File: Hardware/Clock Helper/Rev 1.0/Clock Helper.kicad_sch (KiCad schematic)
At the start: 16 parts, among them J1 IO, SW1 CYCLE/INSTR, SW2 RUN/STOP, SW3 STEP, U1 74HC74

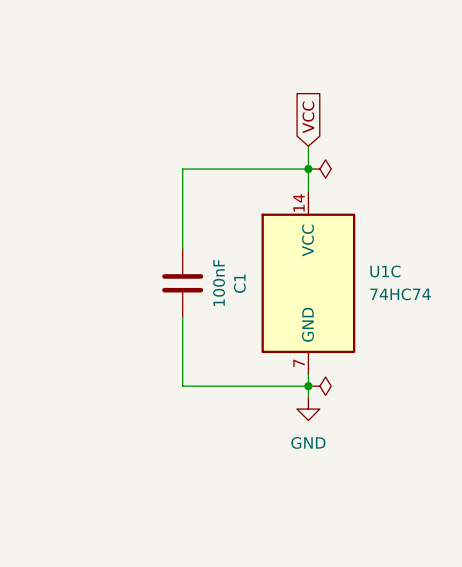
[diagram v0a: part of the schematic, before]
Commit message: Project restructuring
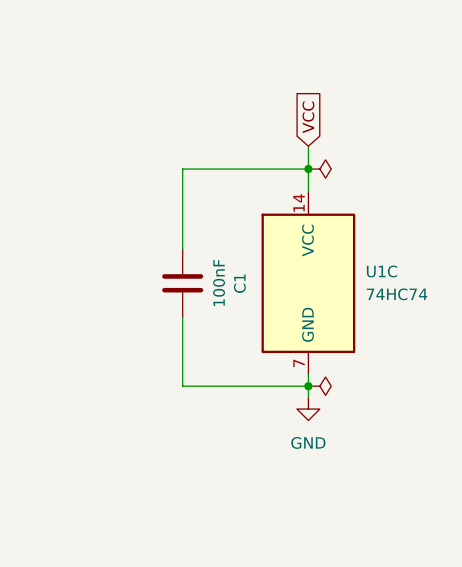
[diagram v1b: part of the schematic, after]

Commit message: Add BOMs
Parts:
- C1: LCSC C49678 -> (none)
- J1: now in the parts list
- R3, R4, R5: LCSC C17513 -> (none)
- SW1, SW2: LCSC (none) -> XKB5858-Z; MPN XKB5858-Z -> (none)
- SW3: LCSC (none) -> XKB5858-W; MPN XKB5858-W -> (none)
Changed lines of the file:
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@@
 			)
 		)
-		(property "LCSC" "C17513"
+		(property "LCSC" ""
 			(at 105.41 76.2 0)
 			(hide yes)
@@
 			)
 		)
-		(property "MPN" "XKB5858-W"
+		(property "LCSC" "XKB5858-W"
 			(at 127 93.98 0)
 			(hide yes)
@@
 			)
 		)
-		(property "LCSC" "C17513"
+		(property "LCSC" ""
 			(at 100.33 82.55 0)
 			(hide yes)
@@
 			)
 		)
-		(property "MPN" "XKB5858-Z"
+		(property "LCSC" "XKB5858-Z"
 			(at 90.17 185.42 0)
 			(hide yes)
@@
 			)
 		)
-		(property "MPN" "XKB5858-Z"
+		(property "LCSC" "XKB5858-Z"
 			(at 172.72 81.28 0)
 			(hide yes)
@@
 		(body_style 1)
 		(exclude_from_sim no)
-		(in_bom no)
+		(in_bom yes)
 		(on_board yes)
 		(in_pos_files yes)
@@
 			)
 		)
-		(property "MPN" "XKB5858-W"
+		(property "LCSC" "XKB5858-W"
 			(at 110.49 185.42 0)
 			(hide yes)
@@
 			)
 		)
-		(property "LCSC" "C17513"
+		(property "LCSC" ""
 			(at 96.52 82.55 0)
 			(hide yes)
@@
 		)
 		(property "Description" "Light emitting diode"
-			(at 91.44 100.33 0)
-			(hide yes)
-			(show_name no)
-			(do_not_autoplace no)
-			(effects
-				(font
-					(size 1.27 1.27)
-				)
-			)
-		)
-		(property "Sim.Pins" "1=K 2=A"
 			(at 91.44 100.33 0)
 			(hide yes)
@@
 			)
 		)
-		(property "LCSC" "C49678"
+		(property "LCSC" ""
 			(at 236.22 146.05 0)
 			(hide yes)
@@
 			)
 		)
-		(property "MPN" "XKB5858-Z"
+		(property "LCSC" "XKB5858-Z"
 			(at 130.81 185.42 0)
 			(hide yes)
@@
 			)
 		)
-		(property "Sim.Pins" "1=K 2=A"
-			(at 186.69 95.25 0)
-			(hide yes)
-			(show_name no)
-			(do_not_autoplace no)
-			(effects
-				(font
-					(size 1.27 1.27)
-				)
-			)
-		)
 		(pin "1"
 		)
@@
 			)
 		)
-		(property "MPN" "XKB5858-Z"
+		(property "LCSC" "XKB5858-Z"
 			(at 127 76.2 0)
 			(hide yes)

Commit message: Add BOMs to README
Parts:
- D1, D2, J1, R1, R2, R3, R4, R5, R6, R7, R8, SW1, SW2, SW3, U1: now left out of the parts list
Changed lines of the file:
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@@
 		(body_style 1)
 		(exclude_from_sim no)
-		(in_bom yes)
+		(in_bom no)
 		(on_board yes)
 		(in_pos_files yes)
@@
 		(body_style 1)
 		(exclude_from_sim no)
-		(in_bom yes)
+		(in_bom no)
 		(on_board yes)
 		(in_pos_files yes)
@@
 		(body_style 1)
 		(exclude_from_sim no)
-		(in_bom yes)
+		(in_bom no)
 		(on_board yes)
 		(in_pos_files yes)
@@
 		(body_style 1)
 		(exclude_from_sim no)
-		(in_bom yes)
+		(in_bom no)
 		(on_board yes)
 		(in_pos_files yes)
@@
 		(body_style 1)
 		(exclude_from_sim no)
-		(in_bom yes)
+		(in_bom no)
 		(on_board yes)
 		(in_pos_files yes)
@@
 		(body_style 1)
 		(exclude_from_sim no)
-		(in_bom yes)
+		(in_bom no)
 		(on_board yes)
 		(in_pos_files yes)
@@
 		(body_style 1)
 		(exclude_from_sim no)
-		(in_bom yes)
+		(in_bom no)
 		(on_board yes)
 		(in_pos_files yes)
@@
 		(body_style 1)
 		(exclude_from_sim no)
-		(in_bom yes)
+		(in_bom no)
 		(on_board yes)
 		(in_pos_files yes)
@@
 		(body_style 1)
 		(exclude_from_sim no)
-		(in_bom yes)
+		(in_bom no)
 		(on_board yes)
 		(in_pos_files yes)
@@
 		(body_style 1)
 		(exclude_from_sim no)
-		(in_bom yes)
+		(in_bom no)
 		(on_board yes)
 		(in_pos_files yes)
@@
 		(body_style 1)
 		(exclude_from_sim no)
-		(in_bom yes)
+		(in_bom no)
 		(on_board yes)
 		(in_pos_files yes)
@@
 		(body_style 1)
 		(exclude_from_sim no)
-		(in_bom yes)
+		(in_bom no)
 		(on_board yes)
 		(in_pos_files yes)
@@
 		(body_style 1)
 		(exclude_from_sim no)
-		(in_bom yes)
+		(in_bom no)
 		(on_board yes)
 		(in_pos_files yes)
@@
 		(body_style 1)
 		(exclude_from_sim no)
-		(in_bom yes)
+		(in_bom no)
 		(on_board yes)
 		(in_pos_files yes)
@@
 		(body_style 1)
 		(exclude_from_sim no)
-		(in_bom yes)
+		(in_bom no)
 		(on_board yes)
 		(in_pos_files yes)
@@
 		(body_style 1)
 		(exclude_from_sim no)
-		(in_bom yes)
+		(in_bom no)
 		(on_board yes)
 		(in_pos_files yes)
@@
 		(body_style 1)
 		(exclude_from_sim no)
-		(in_bom yes)
+		(in_bom no)
 		(on_board yes)
 		(in_pos_files yes)
@@
 		(body_style 1)
 		(exclude_from_sim no)
-		(in_bom yes)
+		(in_bom no)
 		(on_board yes)
 		(in_pos_files yes)
@@
 		(body_style 1)
 		(exclude_from_sim no)
-		(in_bom yes)
+		(in_bom no)
 		(on_board yes)
 		(in_pos_files yes)
@@
 		(body_style 1)
 		(exclude_from_sim no)
-		(in_bom yes)
-		(on_board yes)
-		(in_pos_files yes)
+		(in_bom no)
+		(on_board yes)
+		(in_pos_files yes)
